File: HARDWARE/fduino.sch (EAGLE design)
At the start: 31 parts, among them IC1 DRV8834SMD, Q1 CSM-7X-DU, SW1 SWITCHTHT

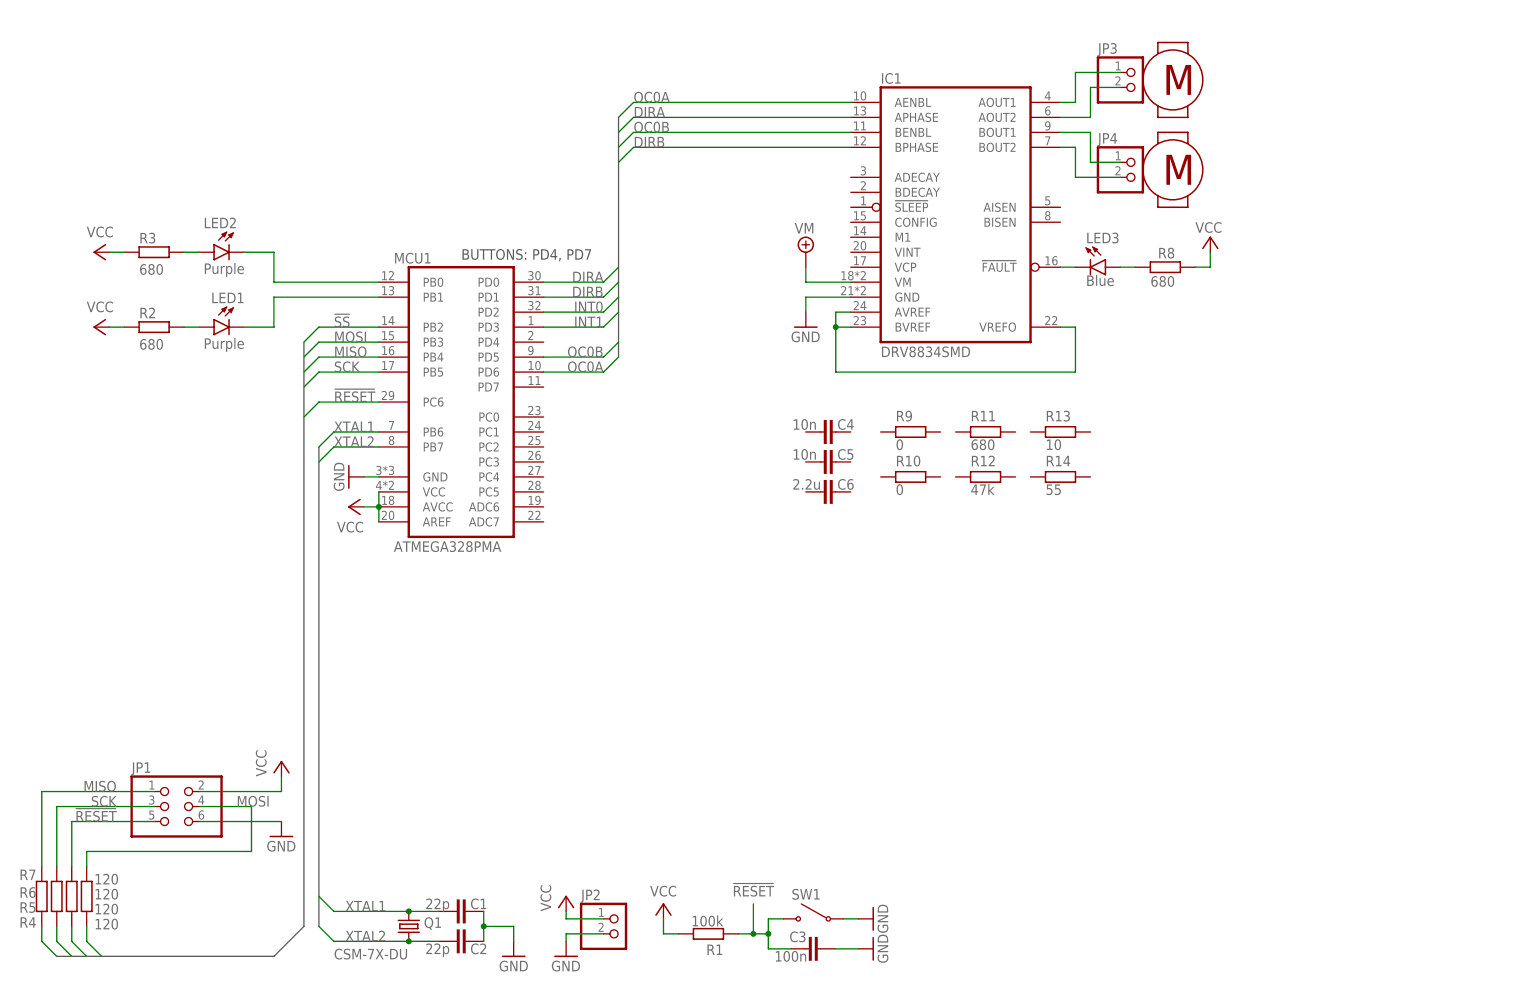
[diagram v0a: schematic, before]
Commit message: common
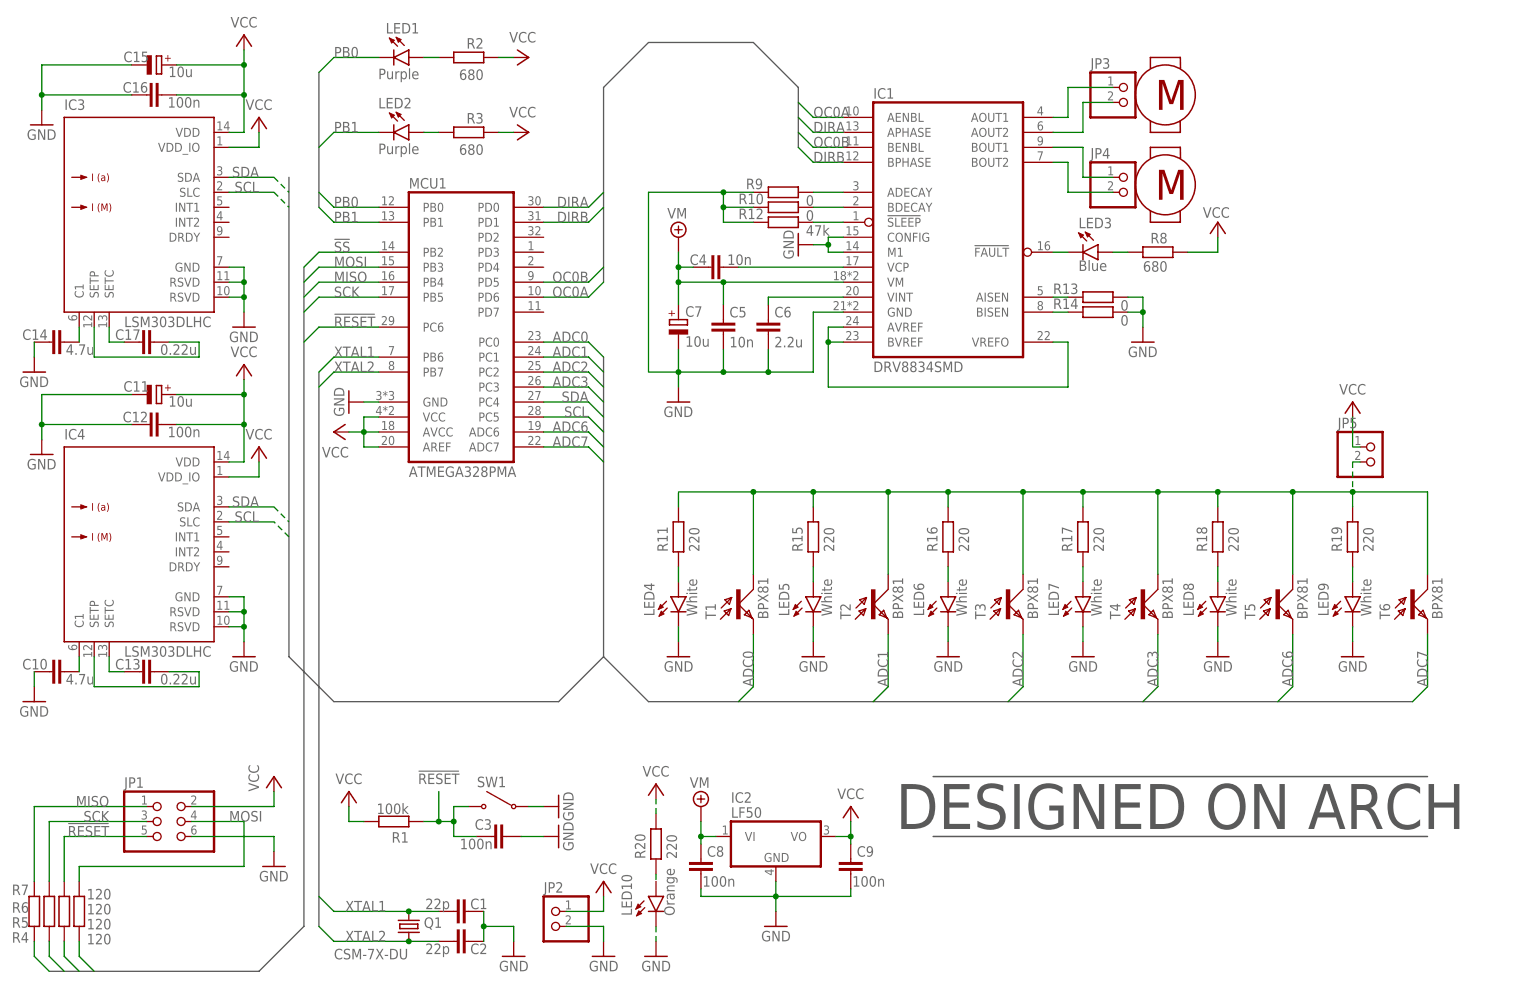
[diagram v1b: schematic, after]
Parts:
- added C10, C14: 4.7u, rcl:C-EUC0603
- added C11, C15, C7: 10u, rcl:CPOL-EUSMCZ
- added C12, C16, C8, C9: 100n, rcl:C-EUC0603
- added C13, C17: 0.22u, rcl:C-EUC0603
- added IC2: LF50, linear:LM340MP-05
- added IC3, IC4: LSM303DLHC, st-microelectronics:LSM303DLHC
- added JP5: (no value), pinhead:PINHD-1X2
- added LED10: Orange, led:LEDSML0603
- added LED4, LED5, LED6, LED7, LED8, LED9: White, led:LEDSML0603
- added R15, R16, R17, R18, R19, R20: 220, rcl:R-EU_R0603
- added T1, T2, T3, T4, T5, T6: BPX81, opto-trans-siemens:BPX81
- R11: value 680 -> 220
- R13: value 10 -> 0
- R14: value 55 -> 0
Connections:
- removed net INT0: MCU1.PD2
- removed net INT1: MCU1.PD3
- new net ADC0: MCU1.PC0, T1.E
- new net ADC1: MCU1.PC1, T2.E
- new net ADC2: MCU1.PC2, T3.E
- new net ADC3: MCU1.PC3, T4.E
- new net ADC6: MCU1.ADC6, T5.E
- new net ADC7: MCU1.ADC7, T6.E
- new net N$14: C4.2, IC1.VCP
- new net N$15: C6.1, IC1.VINT
- new net N$16: IC1.ADECAY, R9.1
- new net N$17: IC1.BDECAY, R10.1
- new net N$18: IC1.!SLEEP, R12.1
- new net N$19: IC1.AISEN, R13.2
- new net N$20: R10.2, R12.2, R9.2
- new net N$21: IC1.BISEN, R14.2
- new net N$22: LED4.A, R11.2
- new net N$23: LED5.A, R15.2
- new net N$24: R15.1
- new net N$26: JP5.2, T1.C, T2.C, T3.C, T4.C, T5.C, T6.C
- new net N$27: LED6.A, R16.2
- new net N$28: R16.1
- new net N$29: C17.2, IC3.SETP
- new net N$30: C17.1, IC3.SETC
- new net N$31: LED7.A, R17.2
- new net N$32: R11.1
- new net N$33: JP5.1
- new net N$35: R17.1
- new net N$36: LED10.A, R20.2
- new net N$37: LED8.A, R18.2
- new net N$38: R18.1
- new net N$40: LED9.A, R19.2
- new net N$41: R19.1
- new net PB0: LED1.C, MCU1.PB0
- new net PB1: LED2.C, MCU1.PB1
- new net SCL: IC3.SLC, IC4.SLC, MCU1.PC5
- new net SDA: IC3.SDA, IC4.SDA, MCU1.PC4
- net GND: now also C10.2, C11.-, C12.1, C14.2, C15.-, C16.1, C5.2, C6.2, C7.-, C8.2, C9.2, IC1.CONFIG, IC1.M1, IC2.GND, IC3.GND, IC3.RSVD@1, IC3.RSVD@2, IC4.GND, IC4.RSVD@1, IC4.RSVD@2, LED10.C, LED4.C, LED5.C, LED6.C, LED7.C, LED8.C, LED9.C, R13.1, R14.1
- net N$1: now also C10.1, IC4.C1; no longer LED1.C
- net N$12: now also C13.1, IC4.SETC; no longer MCU1.PB0
- net N$13: now also C14.1, IC3.C1; no longer MCU1.PB1
- net N$2: now also C13.2, IC4.SETP; no longer LED2.C
- net VCC: now also C11.+, C12.2, C15.+, C16.2, C9.1, IC2.VO, IC3.VDD, IC3.VDD_IO, IC4.VDD, IC4.VDD_IO, R20.1
- net VM: now also C4.1, C5.1, C7.+, C8.1, IC2.VI
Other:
- note added: "Buttons"
- note added: "DESIGNED ON ARCH"
- note added: "Encoders"
- note added: "Line sensors"
- note added: "Motors"
- note added: "Ultra Sonic Sensor"
- note removed: "BUTTONS: PD4, PD7"
- moved on the sheet: C3, C4, C5, C6, IC1, JP1, JP2, JP3, JP4, LED1, LED2, LED3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
